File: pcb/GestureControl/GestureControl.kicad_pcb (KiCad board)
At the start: 4 copper layers, 125.7 x 95.3 mm, 179 parts, among them J1 Conn_01x04_I2I-LCD, J10 EXTERN I2C, J11 Conn_01x02, J12 Conn_01x02, J17 Conn_01x01, J18 Conn_01x01, J19 Conn_01x01, J2 BATT, J3 Conn_01x08, J4 Conn_01x06, J5 Conn_01x10, J6 Conn_01x08, J7 FTDI, J8 Conn_01x06, J9 UART, SW1 SW1, SW2 SW2, U1 AP5100_3.3, U10 VL53L3CXV0DH_RIGHT, U11 VL53L3CXV0DH_LEFT, U12 VL53L3CXV0DH_CENTER, U13 VL53L3CXV0DH_CENTER, U2 AP5100_3.3, U3 VL53L3CXV0DH_CENTER, U4 VL53L3CXV0DH_RIGHT, U5 VL53L3CXV0DH_LEFT, U6 STM32L151RETx, U7 STM32F401RETx, U8 VL53L3CXV0DH_RIGHT, U9 VL53L3CXV0DH_LEFT, Y1 8MHz, Y2 32kHz

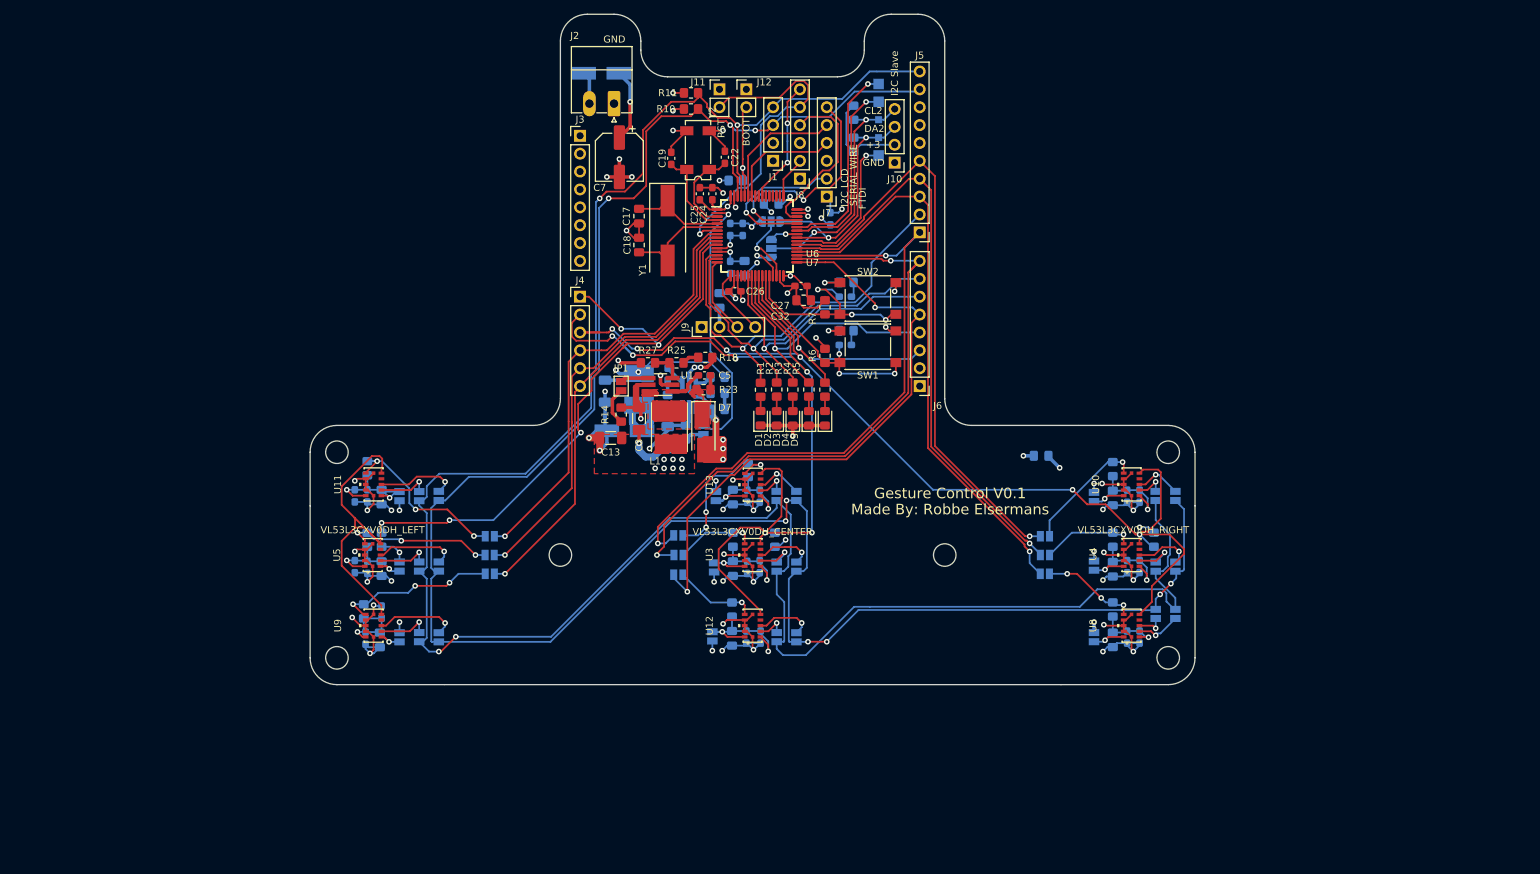
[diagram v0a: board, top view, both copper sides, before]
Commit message: add PCB V12
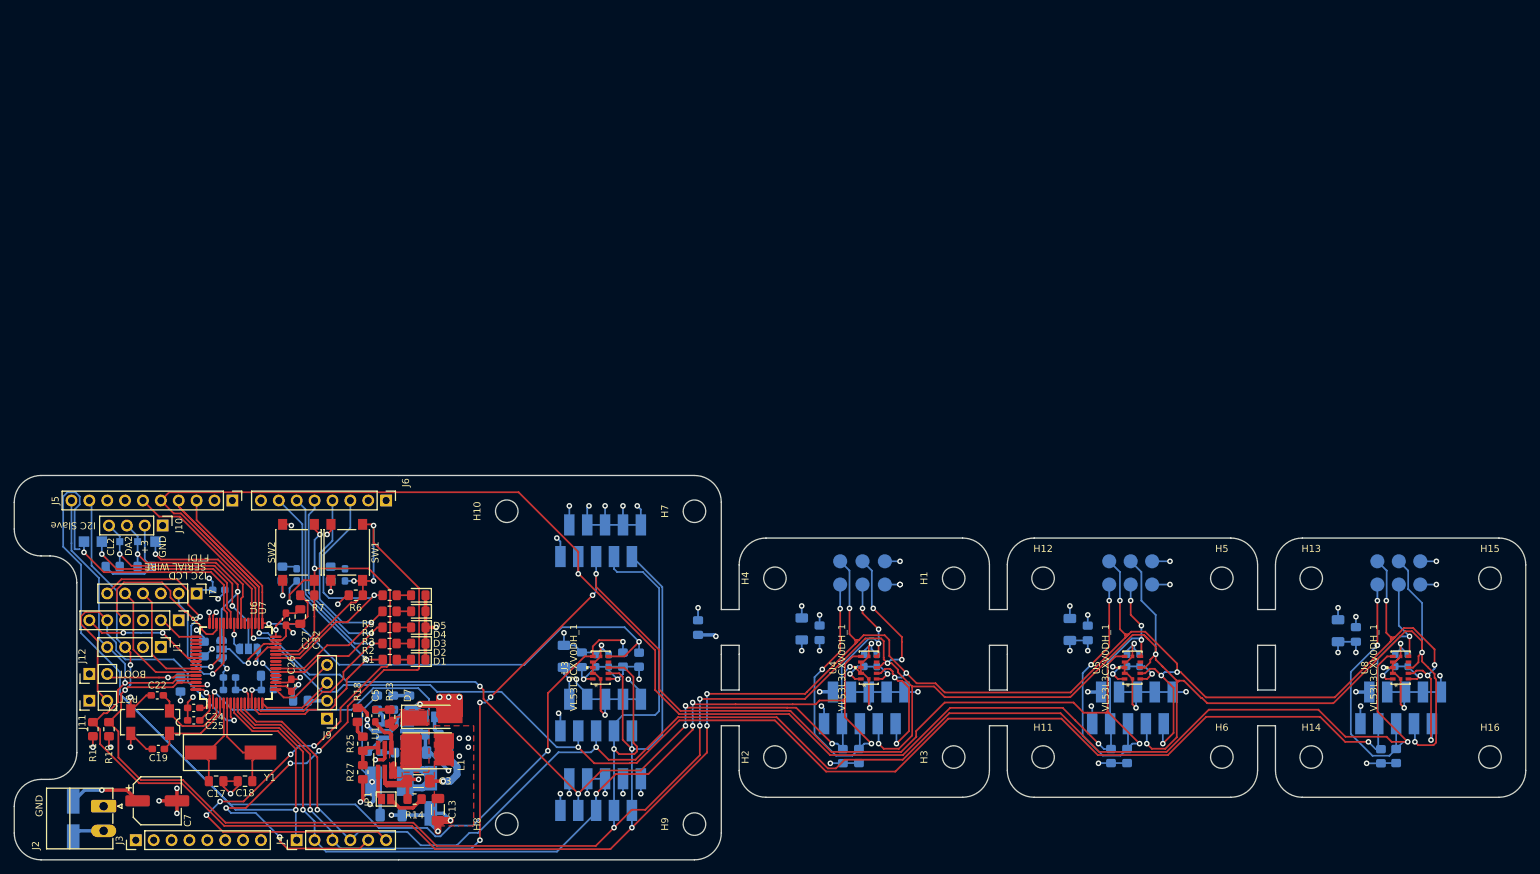
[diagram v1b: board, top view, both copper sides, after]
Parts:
- removed C43, C44, C47, C48, C49, C50, C51, C52: 100n, Capacitor_SMD:C_0603_1608Metric_Pad1.08x0.95mm_HandSolder
- removed C45, C46, C53, C54, C55: 4.7µ, Capacitor_SMD:C_0805_2012Metric_Pad1.18x1.45mm_HandSolder
- removed JP10, JP11, JP12, JP14, JP15, JP16, JP17, JP18, JP19, JP20, JP21, JP22, JP23, JP27, JP28, JP29, JP30, JP31, JP32, JP33, JP34, JP35, JP36, JP37, JP38, JP39, JP40, JP41, JP42, JP43, JP44, JP5, JP6, JP7, JP8, JP9: SolderJumper_2_Open, Jumper:SolderJumper-2_P1.3mm_Open_Pad1.0x1.5mm
- removed R33, R34, R35, R36: 10k, Resistor_SMD:R_0805_2012Metric_Pad1.20x1.40mm_HandSolder
- removed U10: VL53L3CXV0DH_RIGHT, VL53L3CX:VL53L3CXV0DH&slash_1
- removed U11, U9: VL53L3CXV0DH_LEFT, VL53L3CX:VL53L3CXV0DH&slash_1
- removed U12, U13: VL53L3CXV0DH_CENTER, VL53L3CX:VL53L3CXV0DH&slash_1
- added C20: 100n, Capacitor_SMD:C_0603_1608Metric_Pad1.08x0.95mm_HandSolder, B.Cu at (201.4, 129.6)
- added C21: 100n, Capacitor_SMD:C_0603_1608Metric_Pad1.08x0.95mm_HandSolder, B.Cu at (239.5, 129.6)
- added H10: MountingHole, MountingHole:MountingHole_3.2mm_M3, F.Cu at (111.5, 108.5)
- added H11: MountingHole, MountingHole:MountingHole_3.2mm_M3, F.Cu at (187.7, 143.4)
- added H12: MountingHole, MountingHole:MountingHole_3.2mm_M3, F.Cu at (187.7, 118.0)
- added H13: MountingHole, MountingHole:MountingHole_3.2mm_M3, F.Cu at (225.8, 118.0)
- added H14: MountingHole, MountingHole:MountingHole_3.2mm_M3, F.Cu at (225.8, 143.4)
- added H15: MountingHole, MountingHole:MountingHole_3.2mm_M3, F.Cu at (251.2, 118.0)
- added H16: MountingHole, MountingHole:MountingHole_3.2mm_M3, F.Cu at (251.2, 143.4)
- added H7: MountingHole, MountingHole:MountingHole_3.2mm_M3, F.Cu at (138.2, 108.5)
- added H8: MountingHole, MountingHole:MountingHole_3.2mm_M3, F.Cu at (111.5, 152.9)
- added H9: MountingHole, MountingHole:MountingHole_3.2mm_M3, F.Cu at (138.2, 152.9)
- added J13: 690367291076, WR-MM Female SMT Connector:WR-MM_Female_SMT_Connector, B.Cu at (162.3, 136.4)
- added J14: 690367291076, WR-MM Female SMT Connector:WR-MM_Female_SMT_Connector, B.Cu at (200.4, 136.4)
- added J15: 690367291076, WR-MM Female SMT Connector:WR-MM_Female_SMT_Connector, B.Cu at (238.5, 136.4)
- added J16: 690367291076, WR-MM Female SMT Connector:WR-MM_Female_SMT_Connector, B.Cu at (124.8, 148.7)
- added J20: 690367291076, WR-MM Female SMT Connector:WR-MM_Female_SMT_Connector, B.Cu at (124.8, 112.6)
- added J21: 690367291076, WR-MM Female SMT Connector:WR-MM_Female_SMT_Connector, B.Cu at (124.8, 137.4)
- added TP10: TestPoint, TestPoint:TestPoint_Pad_D2.0mm, B.Cu at (200.2, 115.6)
- added TP11: TestPoint, TestPoint:TestPoint_Pad_D2.0mm, B.Cu at (197.1, 118.9)
- added TP12: TestPoint, TestPoint:TestPoint_Pad_D2.0mm, B.Cu at (200.2, 118.9)
- added TP13: TestPoint, TestPoint:TestPoint_Pad_D2.0mm, B.Cu at (203.2, 115.6)
- added TP14: TestPoint, TestPoint:TestPoint_Pad_D2.0mm, B.Cu at (203.2, 118.9)
- added TP15: TestPoint, TestPoint:TestPoint_Pad_D2.0mm, B.Cu at (235.2, 115.6)
- added TP16: TestPoint, TestPoint:TestPoint_Pad_D2.0mm, B.Cu at (238.3, 115.6)
- added TP17: TestPoint, TestPoint:TestPoint_Pad_D2.0mm, B.Cu at (235.2, 118.9)
- added TP18: TestPoint, TestPoint:TestPoint_Pad_D2.0mm, B.Cu at (238.3, 118.9)
- added TP19: TestPoint, TestPoint:TestPoint_Pad_D2.0mm, B.Cu at (241.3, 115.6)
- added TP20: TestPoint, TestPoint:TestPoint_Pad_D2.0mm, B.Cu at (241.3, 118.9)
- added TP3: TestPoint, TestPoint:TestPoint_Pad_D2.0mm, B.Cu at (158.9, 115.6)
- added TP4: TestPoint, TestPoint:TestPoint_Pad_D2.0mm, B.Cu at (162.1, 115.6)
- added TP5: TestPoint, TestPoint:TestPoint_Pad_D2.0mm, B.Cu at (158.9, 118.9)
- added TP6: TestPoint, TestPoint:TestPoint_Pad_D2.0mm, B.Cu at (162.1, 118.9)
- added TP7: TestPoint, TestPoint:TestPoint_Pad_D2.0mm, B.Cu at (165.2, 115.6)
- added TP8: TestPoint, TestPoint:TestPoint_Pad_D2.0mm, B.Cu at (165.2, 118.9)
- added TP9: TestPoint, TestPoint:TestPoint_Pad_D2.0mm, B.Cu at (197.1, 115.6)
- C16: value 4.7µ -> 100n; footprint Capacitor_SMD:C_0805_2012Metric_Pad1.18x1.45mm_HandSolder -> Capacitor_SMD:C_0603_1608Metric_Pad1.08x0.95mm_HandSolder
- C36: value 100n -> 4.7µ; footprint Capacitor_SMD:C_0603_1608Metric_Pad1.08x0.95mm_HandSolder -> Capacitor_SMD:C_0805_2012Metric_Pad1.18x1.45mm_HandSolder
- C39, C40, C41, C42: value 100n -> 10µ; footprint Capacitor_SMD:C_0603_1608Metric_Pad1.08x0.95mm_HandSolder -> Capacitor_SMD:C_1206_3216Metric_Pad1.33x1.80mm_HandSolder
- U3: value VL53L3CXV0DH_CENTER -> VL53L3CXV0DH_1
- U4, U8: value VL53L3CXV0DH_RIGHT -> VL53L3CXV0DH_1
- U5: value VL53L3CXV0DH_LEFT -> VL53L3CXV0DH_1
- moved R17 149.7 mm to (235.7, 143.3)
- moved C15 148.4 mm to (237.7, 129.6), turned to 90 degrees
- moved J19 130.3 mm to (51.4, 112.8), turned to 270 degrees
- moved D6 129.8 mm to (49.9, 152.2), turned to 270 degrees
- moved H5 127.0 mm to (213.1, 118.0)
- moved J18 126.8 mm to (54.0, 112.8), turned to 270 degrees
- moved J12 124.9 mm to (52.2, 131.6), turned to 90 degrees
- moved J11 124.8 mm to (52.2, 135.4), turned to 90 degrees
- moved R11 124.1 mm to (52.7, 139.4), turned to 90 degrees
- moved R22 123.5 mm to (55.5, 116.3), turned to 0 degrees
- moved J2 123.4 mm to (54.2, 150.4), turned to 270 degrees
- moved TP2 123.4 mm to (56.5, 112.8), turned to 270 degrees
- moved R10 120.8 mm to (55.0, 139.4), turned to 90 degrees
- moved TP1 119.9 mm to (59.1, 112.8), turned to 270 degrees
- moved J3 118.3 mm to (58.8, 155.2), turned to 90 degrees
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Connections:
- C10 pad 1: /VL53L3CX center/PWR1 -> +3V3
- C14 pad 1: /VL53L3CX left/PWR1 -> +3V3
- C15 pad 1: /VL53L3CX left/PWR1 -> +3V3
- C16 pad 1: /VL53L3CX left/PWR1 -> +3V3
- C35 pad 1: /VL53L3CX center/PWR0 -> +3V3
- C36 pad 1: /VL53L3CX center/PWR2 -> +3V3
- C37 pad 1: /VL53L3CX center/PWR0 -> +3V3
- C38 pad 1: /VL53L3CX center/PWR2 -> +3V3
- C39 pad 1: /VL53L3CX right/PWR0 -> +3V3
- C40 pad 1: /VL53L3CX right/PWR1 -> +3V3
- C41 pad 1: /VL53L3CX right/PWR2 -> +3V3
- C42 pad 1: /VL53L3CX right/PWR0 -> +3V3
- C8 pad 1: /VL53L3CX center/PWR1 -> +3V3
- C9 pad 1: /VL53L3CX center/PWR1 -> +3V3
- J4 pad 1: GPIOI_0 -> XSHUT_0
- J4 pad 2: GPIOI_1 -> XSHUT_1
- J4 pad 3: GPIOI_2 -> XSHUT_2
- J4 pad 4: _XSHUT_0 -> XSHUT_3
- J4 pad 5: _XSHUT_3 -> SW_1
- J4 pad 6: _XSHUT_6 -> SW_2
- J5 pad 1: _XSHUT_1 -> (no net)
- J5 pad 2: LED_1 -> (no net)
- J5 pad 3: _XSHUT_8 -> GPIOI_0
- J5 pad 4: _XSHUT_5 -> GPIOI_1
- J5 pad 5: _XSHUT_2 -> GPIOI_2
- J5 pad 6: (no net) -> GPIOI_3
- J6 pad 5: _XSHUT_7 -> LED_3
- J6 pad 6: LED_3 -> LED_2
- J6 pad 7: LED_2 -> LED_1
- J6 pad 8: _XSHUT_4 -> (no net)
- R13 pad 1: /VL53L3CX center/PWR0 -> +3V3
- R13 pad 2: XSHUT_1 -> GPIOI_2
- R16 pad 2: GPIOI_0 -> XSHUT_2
- R17 pad 1: /VL53L3CX left/PWR0 -> +3V3
- R17 pad 2: XSHUT_0 -> GPIOI_3
- R29 pad 1: /VL53L3CX center/PWR1 -> +3V3
- R29 pad 2: XSHUT_4 -> XSHUT_1
- R30 pad 1: /VL53L3CX center/PWR2 -> +3V3
- R30 pad 2: XSHUT_7 -> XSHUT_3
- R31 pad 2: GPIOI_2 -> GPIOI_0
- R32 pad 1: /VL53L3CX right/PWR0 -> +3V3
- R32 pad 2: XSHUT_2 -> XSHUT_0
- U3 pad 1: /VL53L3CX center/PWR1 -> +3V3
- U3 pad 10: Net-(JP20-Pad1) -> SCL1
- U3 pad 11: /VL53L3CX center/PWR1 -> +3V3
- U3 pad 5: XSHUT_4 -> XSHUT_0
- U3 pad 7: GPIOI_1 -> GPIOI_0
- U3 pad 9: Net-(JP21-Pad1) -> SDA1
- U4 pad 1: /VL53L3CX right/PWR1 -> +3V3
- U4 pad 10: Net-(JP32-Pad1) -> SCL1
- U4 pad 11: /VL53L3CX right/PWR1 -> +3V3
- U4 pad 5: XSHUT_5 -> XSHUT_1
- U4 pad 7: GPIOI_2 -> GPIOI_1
- U4 pad 9: Net-(JP33-Pad1) -> SDA1
- U5 pad 1: /VL53L3CX left/PWR1 -> +3V3
- U5 pad 10: Net-(JP41-Pad1) -> SCL1
- U5 pad 11: /VL53L3CX left/PWR1 -> +3V3
- U5 pad 5: XSHUT_3 -> XSHUT_2
- U5 pad 7: GPIOI_0 -> GPIOI_2
- U5 pad 9: Net-(JP42-Pad1) -> SDA1
- U6 pad 10: _XSHUT_6 -> XSHUT_2
- U6 pad 11: GPIOI_0 -> XSHUT_3
- U6 pad 24: GPIOI_1 -> (no net)
- U6 pad 25: GPIOI_2 -> (no net)
- U6 pad 33: _XSHUT_7 -> GPIOI_0
- U6 pad 34: _XSHUT_4 -> GPIOI_1
- U6 pad 35: _XSHUT_1 -> GPIOI_2
- U6 pad 36: _XSHUT_8 -> GPIOI_3
- U6 pad 37: _XSHUT_5 -> (no net)
- U6 pad 38: _XSHUT_2 -> (no net)
- U6 pad 8: _XSHUT_0 -> XSHUT_0
- U6 pad 9: _XSHUT_3 -> XSHUT_1
- U7 pad 10: _XSHUT_6 -> XSHUT_2
- U7 pad 11: GPIOI_0 -> XSHUT_3
- U7 pad 24: GPIOI_1 -> (no net)
- U7 pad 25: GPIOI_2 -> (no net)
- U7 pad 33: _XSHUT_7 -> GPIOI_0
- U7 pad 34: _XSHUT_4 -> GPIOI_1
- U7 pad 35: _XSHUT_1 -> GPIOI_2
- U7 pad 36: _XSHUT_8 -> GPIOI_3
- U7 pad 37: _XSHUT_5 -> (no net)
- U7 pad 38: _XSHUT_2 -> (no net)
- U7 pad 8: _XSHUT_0 -> XSHUT_0
- U7 pad 9: _XSHUT_3 -> XSHUT_1
- U8 pad 1: /VL53L3CX right/PWR2 -> +3V3
- U8 pad 10: Net-(JP34-Pad1) -> SCL1
- U8 pad 11: /VL53L3CX right/PWR2 -> +3V3
- U8 pad 5: XSHUT_8 -> XSHUT_3
- U8 pad 7: GPIOI_2 -> GPIOI_3
- U8 pad 9: Net-(JP35-Pad1) -> SDA1
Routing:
- net GPIOI_3: track 0.00 -> 243.2 mm, vias 0 -> 4
- net XSHUT_3: track 21.5 -> 255.7 mm, vias 3 -> 5
- net XSHUT_2: track 17.7 -> 241.2 mm, vias 1 -> 9
- net XSHUT_0: track 26.2 -> 198.5 mm
- net +3V3: track 549.2 -> 700.3 mm, vias 34 -> 48
- net SDA1: track 305.3 -> 455.6 mm, vias 9 -> 14
- net XSHUT_1: track 21.8 -> 170.5 mm, vias 3 -> 7
- net SCL1: track 322.2 -> 440.3 mm, vias 4 -> 17
- net _XSHUT_1: track 90.5 -> 0.00 mm, vias 2 -> 0
- net _XSHUT_4: track 89.3 -> 0.00 mm, vias 2 -> 0
- net SW_2: track 31.7 -> 117.3 mm, vias 3 -> 7
- net _XSHUT_7: track 85.5 -> 0.00 mm, vias 2 -> 0
- net _XSHUT_2: track 84.5 -> 0.00 mm, vias 1 -> 0
- net SW_1: track 31.9 -> 115.2 mm, vias 3 -> 7
- net _XSHUT_5: track 82.4 -> 0.00 mm, vias 1 -> 0
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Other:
- board size 125.7 x 95.3 mm -> 214.8 x 54.6 mm
- board text added: "GND 3V3"
- board text added: "SCL XSHUT"
- board text added: "SDA GPIOI"
- board text removed: "Gesture Control V0.1"
- board text removed: "Made By: Robbe Elsermans"
